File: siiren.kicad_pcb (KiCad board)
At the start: 2 copper layers, 60 x 30 mm, 14 parts, among them J1 USB_C_Receptacle_USB2.0_16P, J2 S2B-PH-SM4-TB(LF)(SN), SW2 K1-1210UN-01, U1 ESP32-C3-WROOM-02, U2 MCP73832-2-OT, U3 USBLC6-2SC6

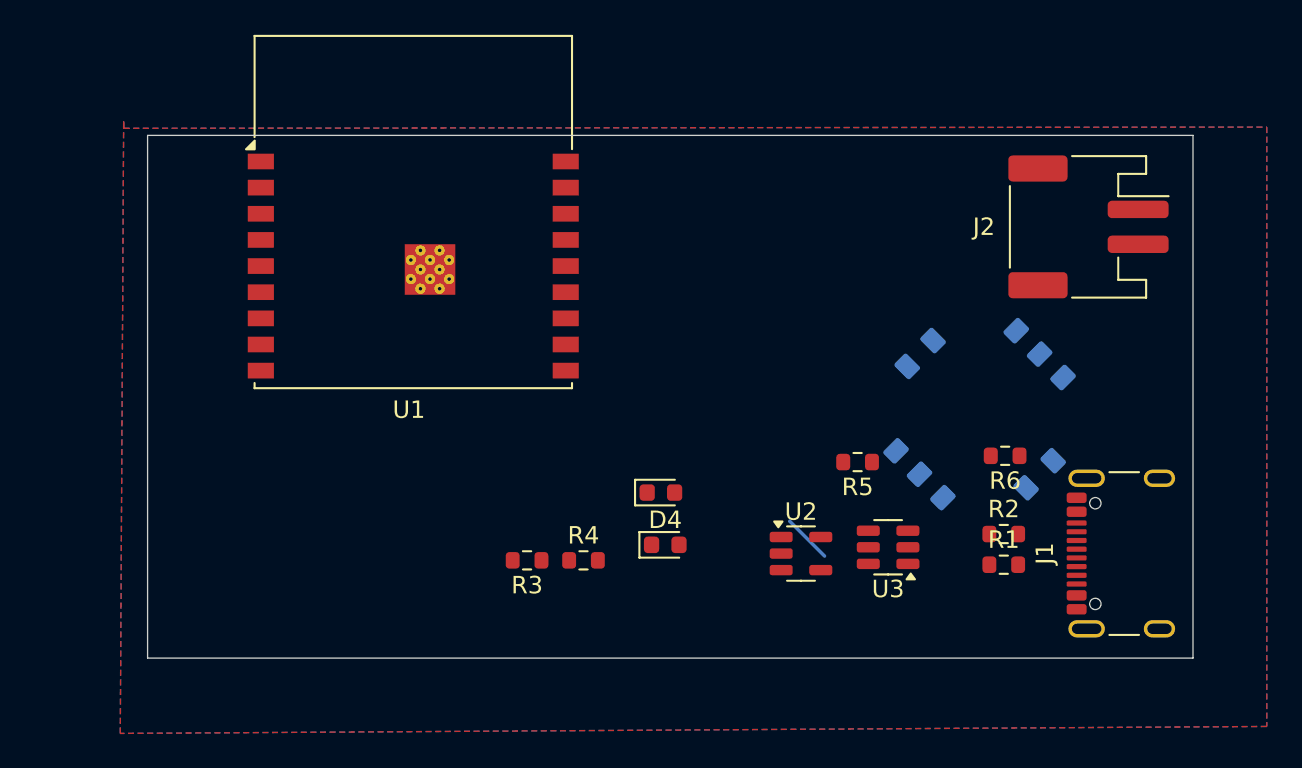
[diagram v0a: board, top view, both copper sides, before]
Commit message: Update image rendering & relayout pcb
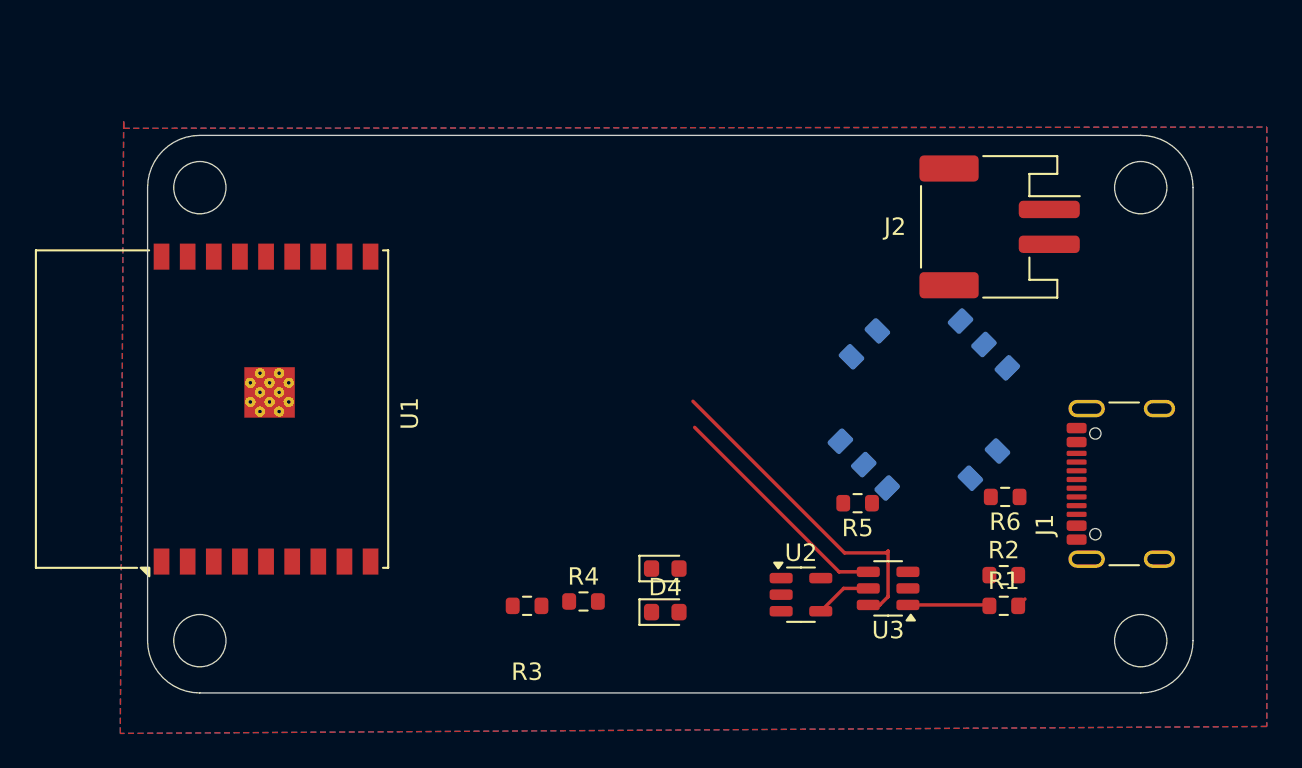
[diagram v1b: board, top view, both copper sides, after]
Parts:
- moved U1 11.8 mm to (36.8, 45.7), turned to 90 degrees
- moved J2 5.10 mm to (78.9, 35.2)
- moved D1 4.37 mm to (59.7, 54.9)
- moved J1 4.00 mm to (87.0, 50.0)
- moved D4 3.86 mm to (59.7, 57.4)
- moved SW2 3.24 mm to (74.6, 45.4)
- moved R3 2.61 mm to (51.8, 57.0)
- moved R1 2.36 mm to (79.1, 57.0)
- moved R2 2.36 mm to (79.1, 55.2)
- moved R4 2.36 mm to (55.0, 56.8)
- moved R5 2.36 mm to (70.8, 51.1)
- moved R6 2.36 mm to (79.2, 50.8)
- moved U2 2.36 mm to (67.5, 56.4)
- moved U3 2.36 mm to (72.5, 56.0)
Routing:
- net /MCU/USB_D+: track 0.00 -> 18.8 mm
- net /MCU/USB_D-: track 0.00 -> 13.4 mm
- net /USB/USB_DP: track 0.00 -> 4.70 mm
- net /USB/USB_D+_RAW: track 0.00 -> 0.55 mm
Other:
- board size 60 x 30 mm -> 60 x 32 mm
